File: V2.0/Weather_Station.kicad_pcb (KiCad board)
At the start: 4 copper layers, 45.2 x 24 mm, 41 parts, among them J1 HS91L02W2C01, J2 TYPE-C16PIN, J3 B-2100S04P-A110, J4 B-2100S04P-A110, J5 ZX-PZ2.54-1-6PZZ, U1 STM32F103C8T6, U2 HDC1080DMBR, U3 AMS1117-3.3, U5 SRV05-4, Y1 X322516MLB4SI

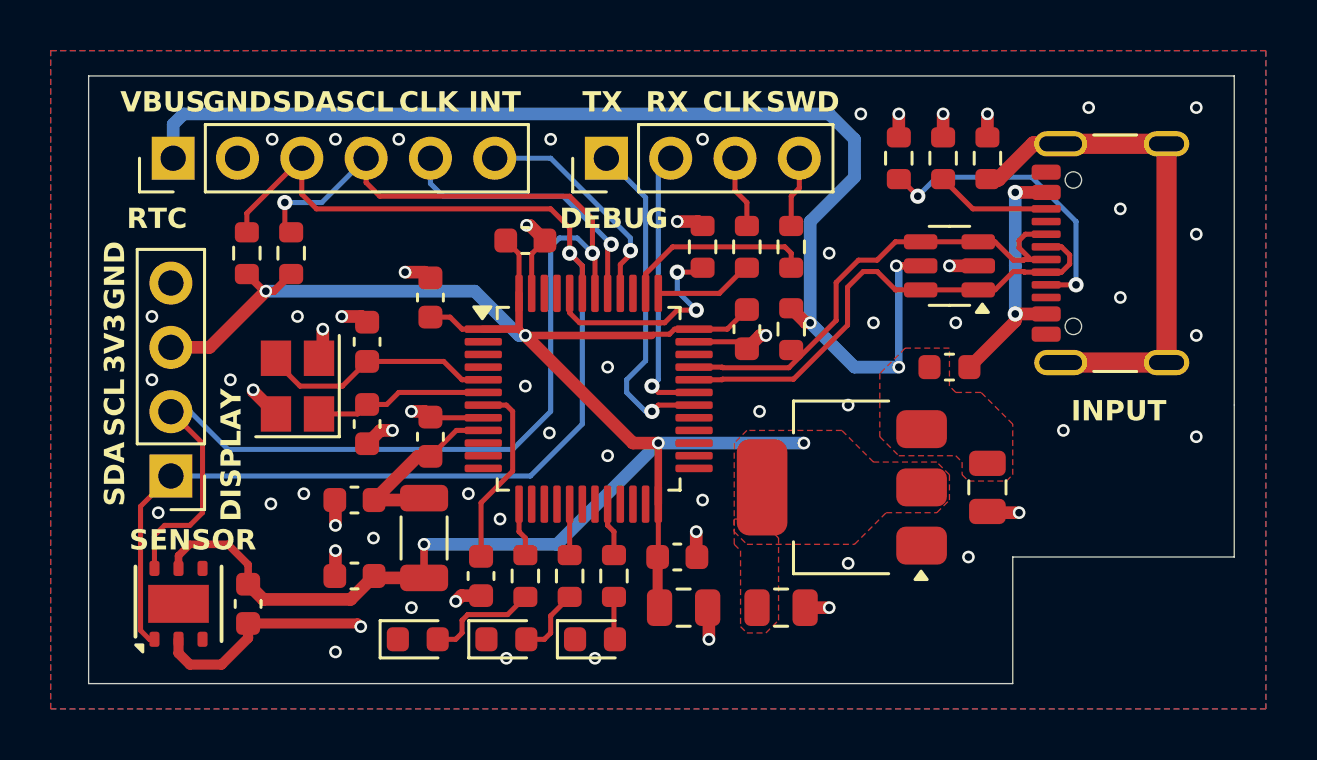
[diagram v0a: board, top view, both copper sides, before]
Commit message: V2 should be finished!!
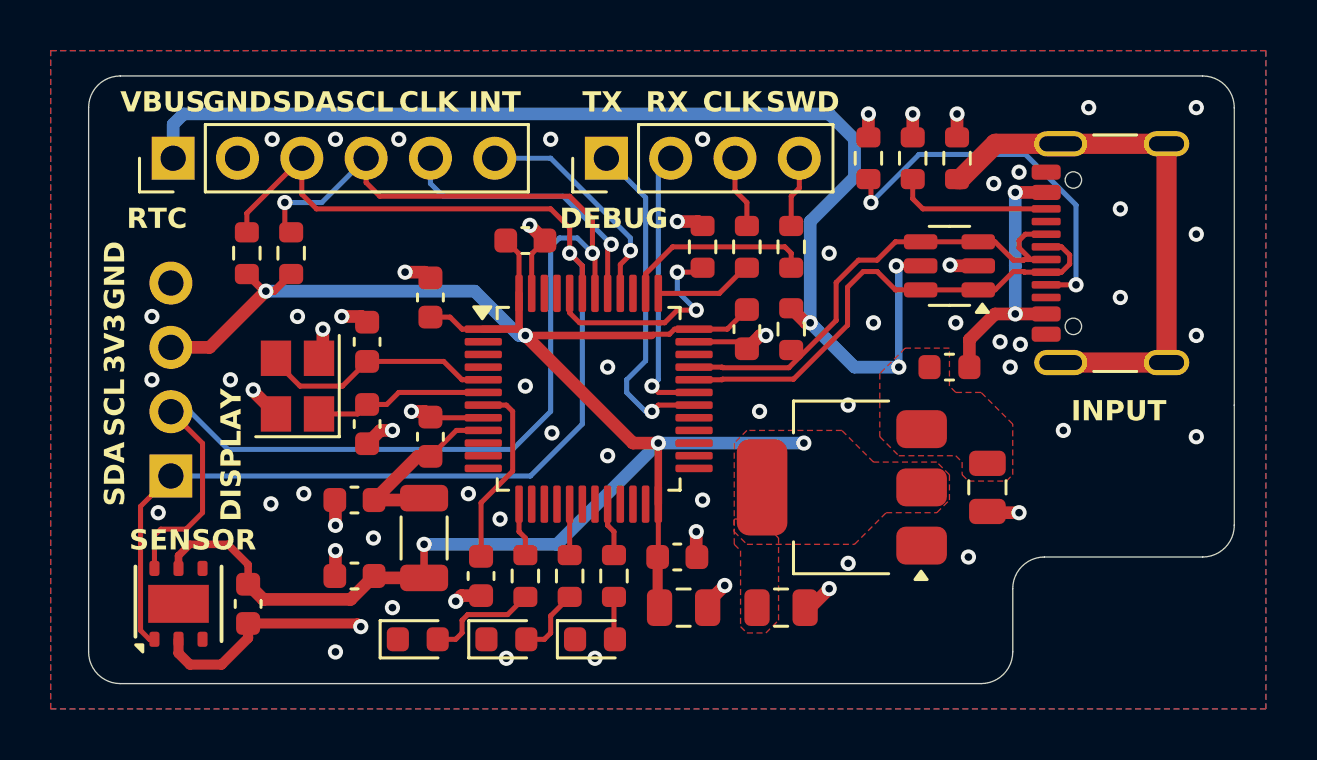
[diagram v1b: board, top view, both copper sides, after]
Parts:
- added G***: LOGO, LOGO, B.Cu at (206.1, 100.5)
- J3: moved to B.Cu
- moved R4 1.20 mm to (202.3, 82.2)
- moved R5 1.20 mm to (204.1, 82.2)
- moved R9 1.20 mm to (205.8, 82.2)
- turned J3 to 0 degrees
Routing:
- net /CC1: track 12.0 -> 15.0 mm
- net /CC2: track 4.56 -> 6.21 mm
- net /Shield: track 20.5 -> 21.7 mm
- net GND: track 36.9 -> 37.0 mm, vias 61 -> 65
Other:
- outline, holes or cut-outs redrawn
- board text added: "Weather Station V2.0"
